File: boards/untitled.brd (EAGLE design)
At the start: 76.2 x 49.5 mm, 36 parts, among them IC1 ULN2004AN

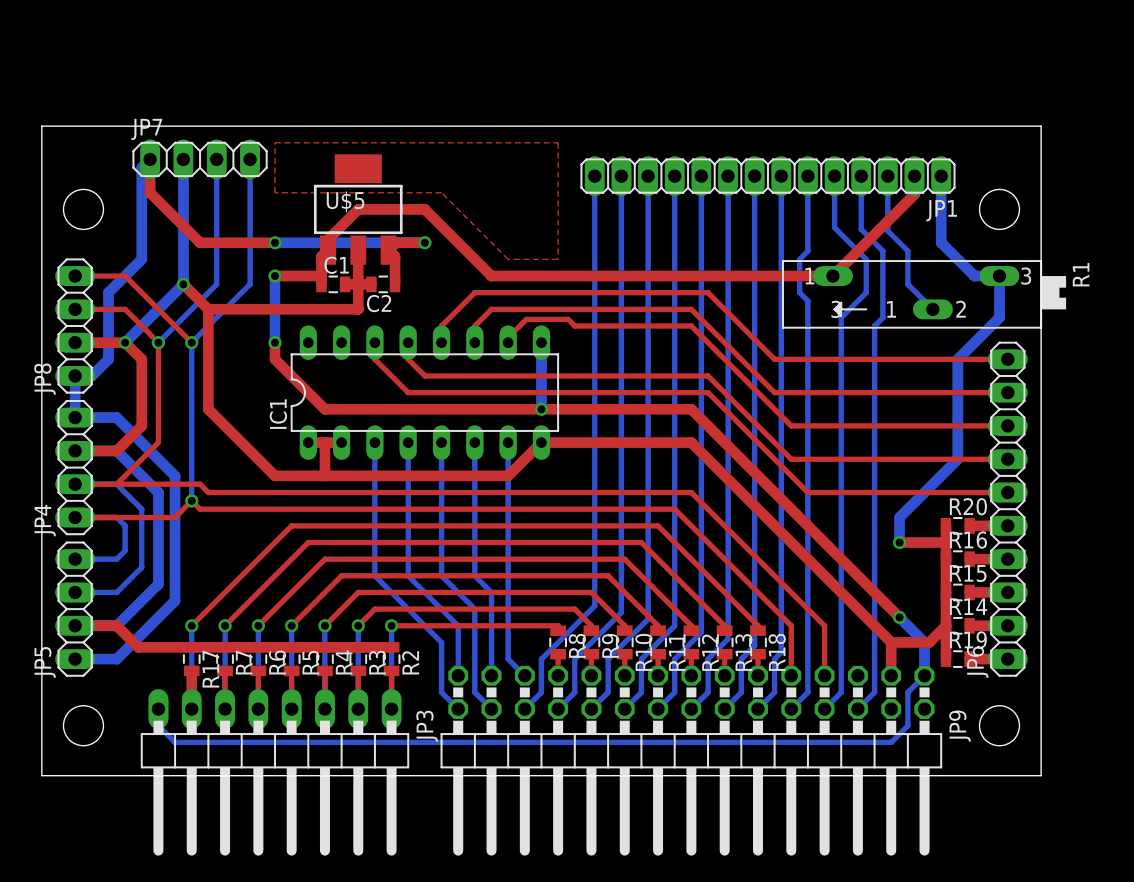
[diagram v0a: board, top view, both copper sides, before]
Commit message: put all the downloaded files into directories
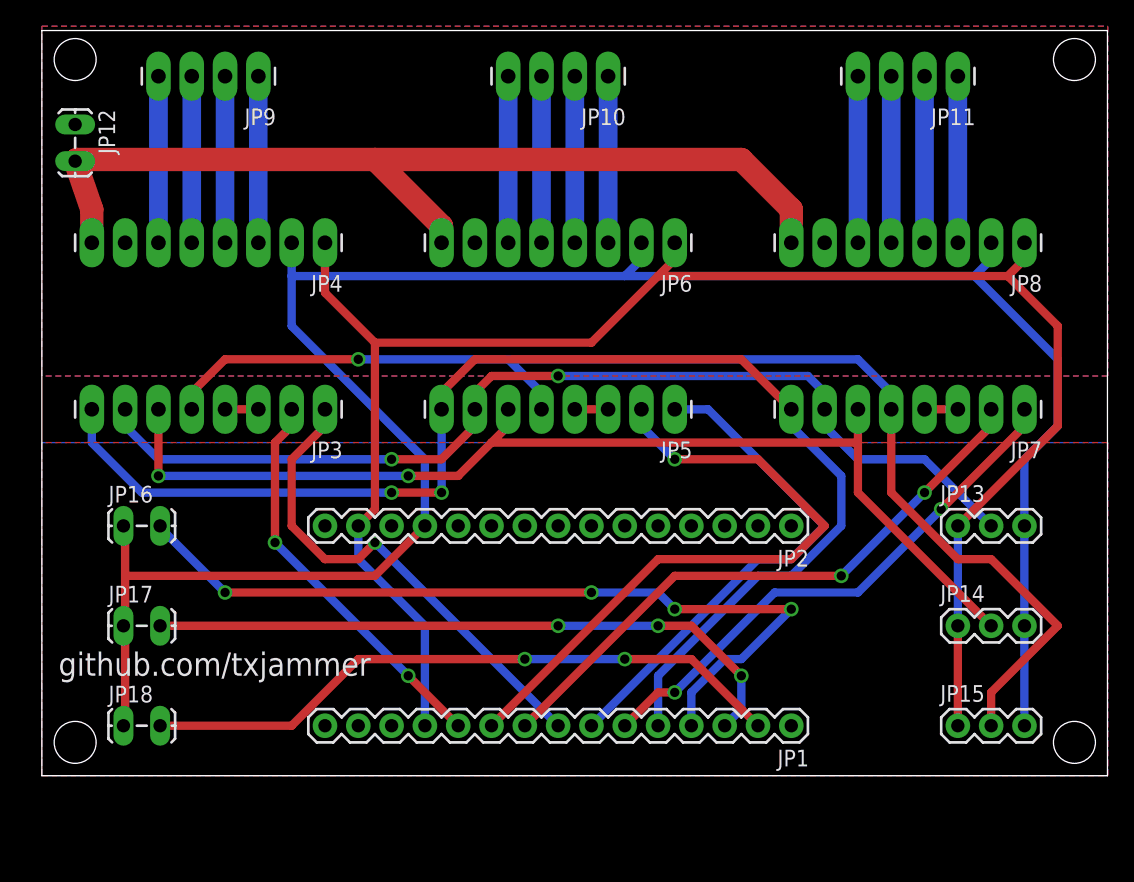
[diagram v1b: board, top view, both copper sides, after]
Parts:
- removed C1, C2, R10, R11, R12, R13, R14, R15, R16, R17, R18, R19, R2, R20, R3, R4, R5, R6, R7, R8, R9: (no value), ASL:0805
- removed IC1: ULN2004AN, uln-udn:DIL16
- removed R1: (no value), pot:SP19L
- removed U$1, U$2, U$3, U$4: (no value), ASL:STAND-OFF-TIGHT
- removed U$5: LM3940IMP-3.3, LM3940:SOT223
- added JP10, JP11: (no value), SparkFun:1X04_LONGPADS
- added JP12, JP16, JP17, JP18: (no value), SparkFun:1X02_LOCK_LONGPADS
- added JP13, JP14, JP15: (no value), SparkFun:1X03
- added JP2: M15, SparkFun:1X15
- JP1: value (none) -> M15; device pinhead_non_standard:1X14 -> SparkFun:1X15
- JP3: device pinhead:1X08/90 -> SparkFun:1X08_LONGPADS
- JP4, JP5, JP7, JP8: device pinhead_non_standard:1X04 -> SparkFun:1X08_LONGPADS
- JP6: device pinhead:1X10 -> SparkFun:1X08_LONGPADS
- JP9: device pinhead:2X15/90 -> SparkFun:1X04_LONGPADS
- moved JP8 72.7 mm to (74.9, 40.6), turned to 180 degrees
- moved JP7 66.3 mm to (74.9, 27.9), turned to 180 degrees
- moved JP9 61.7 mm to (16.5, 53.3)
- moved JP5 48.4 mm to (48.3, 27.9), turned to 180 degrees
- moved JP1 42.2 mm to (57.1, 3.81)
- moved JP6 32.5 mm to (48.3, 40.6), turned to 180 degrees
- moved JP3 26.9 mm to (21.6, 27.9)
- moved JP4 26.1 mm to (21.6, 40.6), turned to 180 degrees
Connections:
- removed net 3.3V: C2.1, JP4.4, JP5.1, JP7.1, JP8.1, U$5.3
- removed net N$16: JP3.4, R11.1, R5.2
- removed net N$17: JP3.5, R12.1, R6.2
- removed net N$18: JP3.6, R13.1, R7.2
- removed net N$19: JP9.13, R13.2
- removed net N$20: JP9.15, R12.2
- removed net N$21: JP9.17, R11.2
- removed net N$22: JP9.19, R10.2
- removed net N$23: JP9.21, R9.2
- removed net N$24: JP9.23, R8.2
- removed net N$25: JP1.14, JP9.26
- removed net N$26: JP3.7, R17.2, R18.1
- removed net N$27: IC1.7, JP9.25
- removed net N$28: JP6.2, R14.2
- removed net N$29: JP6.3, R15.2
- removed net N$30: JP6.4, R16.2
- removed net N$31: IC1.12, JP6.10
- removed net N$32: IC1.5, JP9.28
- removed net N$33: JP4.2, JP5.3, JP7.3, JP8.3, JP9.7
- removed net N$35: JP9.11, R18.2
- removed net N$36: JP6.1, R19.2
- removed net N$37: JP6.5, R20.2
- removed net N$38: IC1.4, JP9.29
- removed net N$39: IC1.3, JP9.30
- removed net N$40: IC1.10, JP6.8
- removed net N$41: IC1.11, JP6.9
- removed net N$43: IC1.13, JP6.7
- removed net N$44: IC1.14, JP6.6
- removed net N$46: IC1.6, JP9.27
- removed net VCC: C1.1, IC1.9, JP1.2, JP3.8, JP9.1, R1.A, U$5.1
- new net 5V: JP13.3, JP14.3, JP15.3, JP16.1, JP17.1, JP18.1, JP2.12, JP4.2, JP6.2, JP8.2
- new net DISABLE: JP1.5, JP3.8, JP5.8, JP7.8
- new net GNDMOT: JP12.1, JP4.7, JP6.7, JP8.7
- new net MS1: JP13.2, JP3.7, JP5.7, JP7.7
- new net MS2: JP14.2, JP3.6, JP5.6, JP7.6
- new net MS3: JP15.2, JP3.5, JP5.5, JP7.5
- new net SPINDLE_EN: JP1.1
- new net SPIN_DIR: JP2.1
- new net VMOT: JP12.2, JP4.8, JP6.8, JP8.8
- new net XDIR: JP1.8, JP3.1
- new net XLIM: JP1.4, JP16.2
- new net XSTP: JP1.11, JP3.2
- new net YDIR: JP1.7, JP5.1
- new net YLIM: JP1.3, JP17.2
- new net YSTP: JP1.10, JP5.2
- new net ZDIR: JP1.6, JP7.1
- new net ZLIM: JP1.2, JP18.2
- new net ZSTP: JP1.9, JP7.2
- net GND: now also JP1.12, JP13.1, JP14.1, JP15.1, JP2.14, JP4.1, JP6.1, JP8.1; no longer C1.2, C2.2, IC1.1, IC1.2, IC1.8, JP1.1, JP4.3, JP5.2, JP7.2, JP8.2, JP9.3, R1.E, R14.1, R15.1, R16.1, R17.1, R19.1, R2.1, R20.1, R3.1, R4.1, R5.1, R6.1, R7.1, U$5.2
- net N$1: now also JP5.3, JP5.4; no longer JP1.3, R1.S
- net N$10: now also JP10.4, JP6.6; no longer JP1.9, JP9.16
- net N$11: now also JP10.3, JP6.5; no longer JP1.10, JP9.18
- net N$12: now also JP10.2, JP6.4; no longer JP1.11, JP9.20
- net N$13: now also JP10.1, JP6.3; no longer JP1.12, JP9.22
- net N$14: now also JP7.3, JP7.4; no longer JP1.13, JP9.24
- net N$15: now also JP3.4; no longer R10.1, R4.2
- net N$2: now also JP4.6, JP9.4; no longer JP3.1, R2.2, R8.1
- net N$3: now also JP4.5, JP9.3; no longer JP3.2, R3.2, R9.1
- net N$4: now also JP4.4, JP9.2; no longer JP1.4, JP9.6
- net N$5: now also JP4.3, JP9.1; no longer JP1.5, JP9.8
- net N$6: now also JP11.4, JP8.6; no longer JP1.6, JP9.10
- net N$7: now also JP11.3, JP8.5; no longer JP1.7, JP9.12
- net N$8: now also JP11.2; no longer JP4.1, JP5.4, JP7.4, JP9.9
- net N$9: now also JP11.1, JP8.3; no longer JP1.8, JP9.14
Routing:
- net VCC: track 195.4 -> 0.00 mm, vias 4 -> 0
- net 5V: track 0.00 -> 162.0 mm
- net N$33: track 116.9 -> 0.00 mm, vias 1 -> 0
- net N$8: track 115.0 -> 12.7 mm, vias 2 -> 0
- net DISABLE: track 0.00 -> 100.7 mm, vias 0 -> 2
- net MS3: track 0.00 -> 95.8 mm, vias 0 -> 1
- net GND: track 229.4 -> 136.6 mm, vias 3 -> 0
- net MS2: track 0.00 -> 83.3 mm, vias 0 -> 2
- net 3.3V: track 82.1 -> 0.00 mm, vias 2 -> 0
- net MS1: track 0.00 -> 78.7 mm, vias 0 -> 2
- net VMOT: track 0.00 -> 73.7 mm
- net XLIM: track 0.00 -> 63.8 mm, vias 0 -> 4
- net N$26: track 59.1 -> 0.00 mm, vias 1 -> 0
- net N$44: track 53.7 -> 0.00 mm
- net N$18: track 53.0 -> 0.00 mm, vias 1 -> 0
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- added copper zone on layer 1, net GND
- added copper zone on layer 16, net GND
- added copper zone on layer 1, net GNDMOT
- added copper zone on layer 16, net GNDMOT
- removed copper zone on layer 1, net N$34
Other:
- board size 76.2 x 49.5 mm -> 81.3 x 56.8 mm
- board text added: "github.com/txjammer"
